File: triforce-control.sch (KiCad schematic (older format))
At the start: 21 parts, among them U1 ADAFRUIT_HUZZAH, U2 bno055, U3 LPC1768

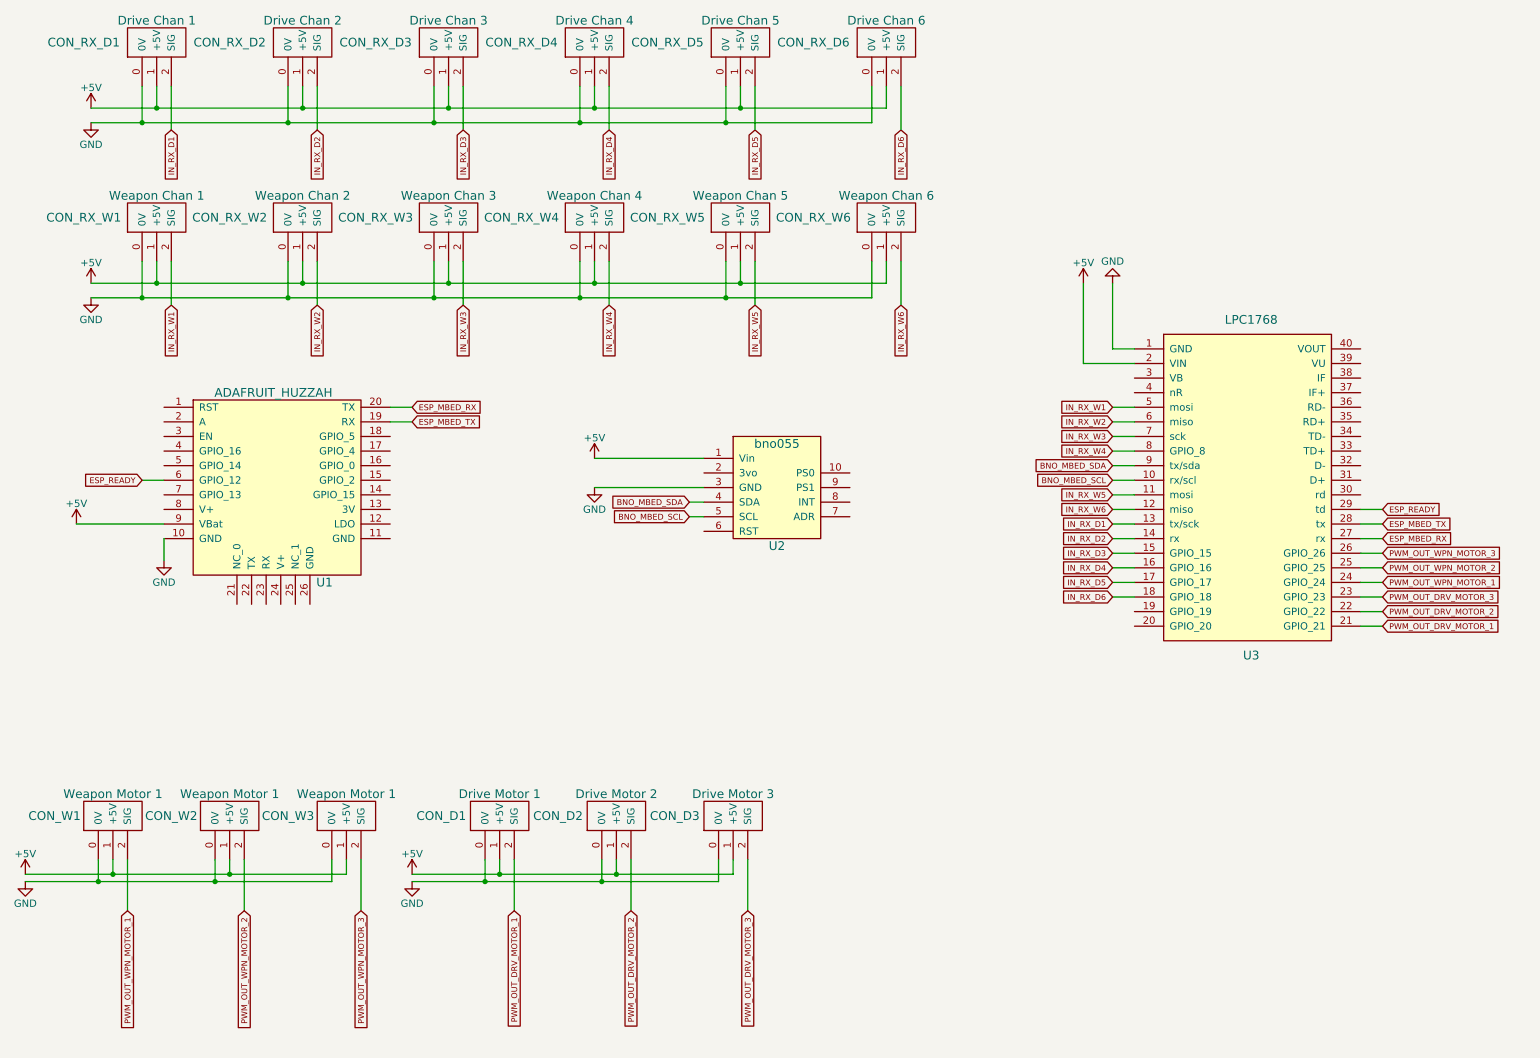
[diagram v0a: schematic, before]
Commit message: Started new PCB design.
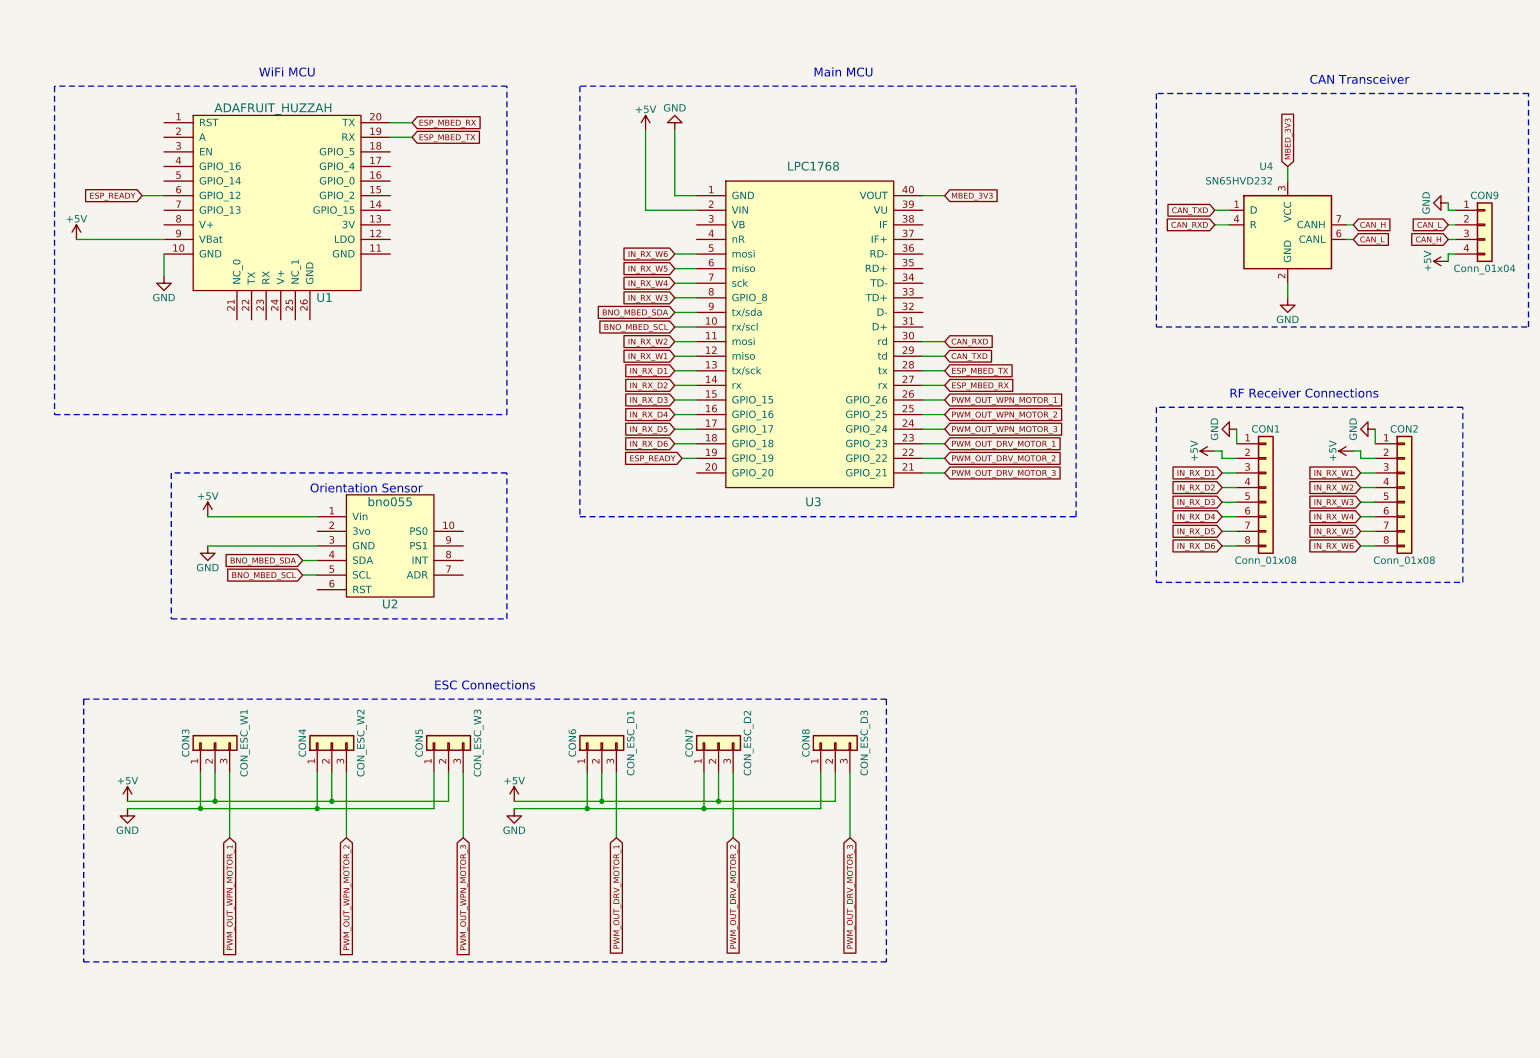
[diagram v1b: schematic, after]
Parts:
- removed CON_D1: Drive Motor 1, mbed:AngledServoCon, symbol Servo
- removed CON_D2: Drive Motor 2, mbed:AngledServoCon, symbol Servo
- removed CON_D3: Drive Motor 3, mbed:AngledServoCon, symbol Servo
- removed CON_RX_D1: Drive Chan 1, mbed:AngledServoCon, symbol Servo
- removed CON_RX_D2: Drive Chan 2, mbed:AngledServoCon, symbol Servo
- removed CON_RX_D3: Drive Chan 3, mbed:AngledServoCon, symbol Servo
- removed CON_RX_D4: Drive Chan 4, mbed:AngledServoCon, symbol Servo
- removed CON_RX_D5: Drive Chan 5, mbed:AngledServoCon, symbol Servo
- removed CON_RX_D6: Drive Chan 6, mbed:AngledServoCon, symbol Servo
- removed CON_RX_W1: Weapon Chan 1, mbed:AngledServoCon, symbol Servo
- removed CON_RX_W2: Weapon Chan 2, mbed:AngledServoCon, symbol Servo
- removed CON_RX_W3: Weapon Chan 3, mbed:AngledServoCon, symbol Servo
- removed CON_RX_W4: Weapon Chan 4, mbed:AngledServoCon, symbol Servo
- removed CON_RX_W5: Weapon Chan 5, mbed:AngledServoCon, symbol Servo
- removed CON_RX_W6: Weapon Chan 6, mbed:AngledServoCon, symbol Servo
- removed CON_W1, CON_W2, CON_W3: Weapon Motor 1, mbed:AngledServoCon, symbol Servo
- added CON1, CON2: Conn_01x08, Connectors_JST:JST_PH_S8B-PH-K_08x2.00mm_Angled, symbol Conn_01x08
- added CON3: CON_ESC_W1, mbed:Pin_Header_Angled_3x01_Pitch2.54mm, symbol Conn_01x03
- added CON4: CON_ESC_W2, mbed:Pin_Header_Angled_3x01_Pitch2.54mm, symbol Conn_01x03
- added CON5: CON_ESC_W3, mbed:Pin_Header_Angled_3x01_Pitch2.54mm, symbol Conn_01x03
- added CON6: CON_ESC_D1, mbed:Pin_Header_Angled_3x01_Pitch2.54mm, symbol Conn_01x03
- added CON7: CON_ESC_D2, mbed:Pin_Header_Angled_3x01_Pitch2.54mm, symbol Conn_01x03
- added CON8: CON_ESC_D3, mbed:Pin_Header_Angled_3x01_Pitch2.54mm, symbol Conn_01x03
- added CON9: Conn_01x04, Connectors_JST:JST_PH_S4B-PH-K_04x2.00mm_Angled, symbol Conn_01x04
- added U4: SN65HVD232, Housings_SOIC:SOIC-8_3.9x4.9mm_Pitch1.27mm, symbol SN65HVD232
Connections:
- net +5V: now also CON1.2 (Pin_2), CON2.2 (Pin_2), CON3.2 (Pin_2), CON4.2 (Pin_2), CON5.2 (Pin_2), CON6.2 (Pin_2), CON7.2 (Pin_2), CON8.2 (Pin_2), CON9.4 (Pin_4)
- net ESP_READY: now also U3.19 (GPIO_19); no longer U3.29 (td)
- net GND: now also CON1.1 (Pin_1), CON2.1 (Pin_1), CON3.1 (Pin_1), CON4.1 (Pin_1), CON5.1 (Pin_1), CON6.1 (Pin_1), CON7.1 (Pin_1), CON8.1 (Pin_1), CON9.1 (Pin_1), U4.2 (GND)
- net IN_RX_D1: now also CON1.3 (Pin_3)
- net IN_RX_D2: now also CON1.4 (Pin_4)
- net IN_RX_D3: now also CON1.5 (Pin_5)
- net IN_RX_D4: now also CON1.6 (Pin_6)
- net IN_RX_D5: now also CON1.7 (Pin_7)
- net IN_RX_D6: now also CON1.8 (Pin_8)
- net IN_RX_W1: now also U3.12 (miso), CON2.3 (Pin_3); no longer U3.5 (mosi)
- net IN_RX_W2: now also U3.11 (mosi), CON2.4 (Pin_4); no longer U3.6 (miso)
- net IN_RX_W3: now also U3.8 (GPIO_8), CON2.5 (Pin_5); no longer U3.7 (sck)
- net IN_RX_W4: now also U3.7 (sck), CON2.6 (Pin_6); no longer U3.8 (GPIO_8)
- net IN_RX_W5: now also U3.6 (miso), CON2.7 (Pin_7); no longer U3.11 (mosi)
- net IN_RX_W6: now also U3.5 (mosi), CON2.8 (Pin_8); no longer U3.12 (miso)
- net PWM_OUT_DRV_MOTOR_1: now also U3.23 (GPIO_23), CON6.3 (Pin_3); no longer U3.21 (GPIO_21)
- net PWM_OUT_DRV_MOTOR_2: now also CON7.3 (Pin_3)
- net PWM_OUT_DRV_MOTOR_3: now also U3.21 (GPIO_21), CON8.3 (Pin_3); no longer U3.23 (GPIO_23)
- net PWM_OUT_WPN_MOTOR_1: now also U3.26 (GPIO_26), CON3.3 (Pin_3); no longer U3.24 (GPIO_24)
- net PWM_OUT_WPN_MOTOR_2: now also CON4.3 (Pin_3)
- net PWM_OUT_WPN_MOTOR_3: now also U3.24 (GPIO_24), CON5.3 (Pin_3); no longer U3.26 (GPIO_26)
- net CAN_RXD: now reaches U3.30 (rd)
- net CAN_RXD: now also U4.4 (R)
- net MBED_3V3: now reaches U3.40 (VOUT)
- net MBED_3V3: now also U4.3 (VCC)
- new net CAN_H: CON9.3 (Pin_3), U4.7 (CANH)
- new net CAN_L: CON9.2 (Pin_2), U4.6 (CANL)
- new net CAN_TXD: U3.29 (td), U4.1 (D)
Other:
- note added: "CAN Transceiver"
- note added: "ESC Connections"
- note added: "Main MCU"
- note added: "Orientation Sensor"
- note added: "RF Receiver Connections"
- note added: "WiFi MCU"
- moved on the sheet: U1, U2, U3
